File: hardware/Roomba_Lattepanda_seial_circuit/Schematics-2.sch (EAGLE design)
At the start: 14 parts

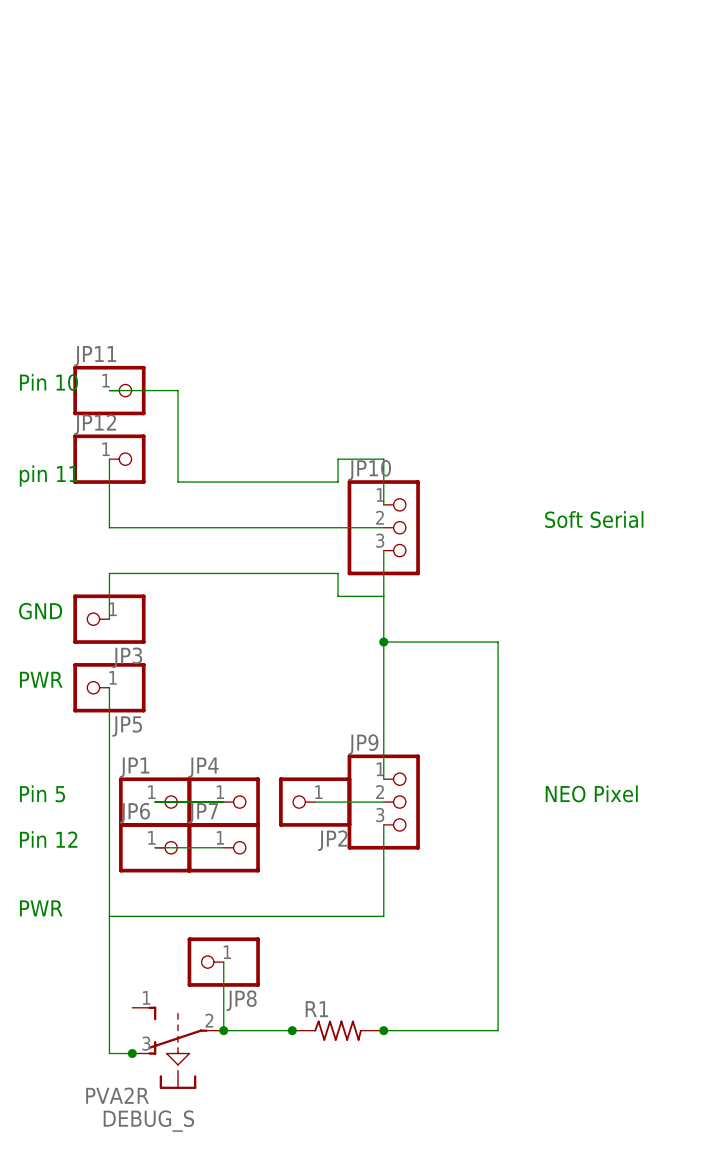
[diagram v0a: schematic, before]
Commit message: update hardware
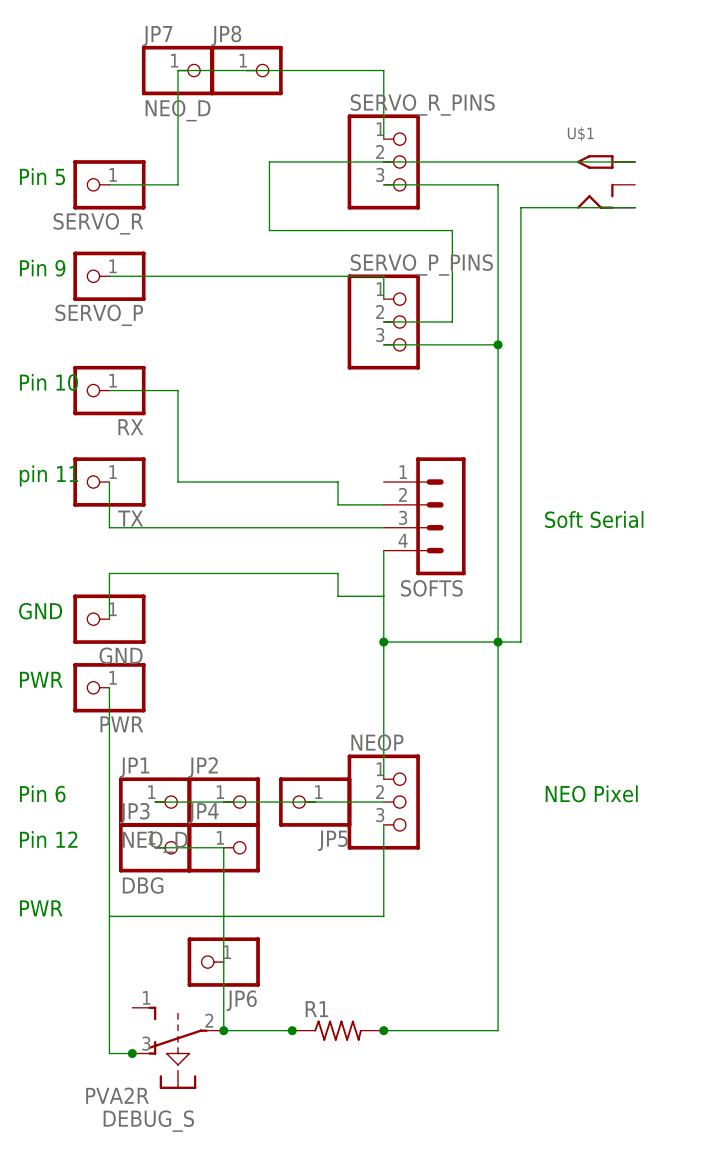
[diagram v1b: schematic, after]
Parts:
- removed JP10: (no value), adafruit:PINHD-1X3CB
- removed JP11, JP12: (no value), adafruit:PINHD-1X1
- added GND, PWR, RX, SERVO_P, SERVO_R, TX: (no value), adafruit:PINHD-1X1CB
- added SERVO_P_PINS, SERVO_R_PINS: (no value), adafruit:PINHD-1X3CB
- added SOFTS: (no value), con-lstb:MA04-1
- added U$1: 2.1MMJACKTHM, adafruit:2.1MMJACKTHM
- JP1, JP7: value (none) -> NEO_D
- JP3: value (none) -> DBG
- renumbered JP9 to NEOP
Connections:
- removed net N$6: DEBUG_S1.P, JP8.1, R1.1
- removed net N$7: JP2.1, NEOP.2
- new net N$10: JP7.1, JP8.1, SERVO_R.1, SERVO_R_PINS.1
- new net N$12: SERVO_P.1, SERVO_P_PINS.1
- new net N$9: SERVO_P_PINS.2, SERVO_R_PINS.2, U$1.TIP
- net N$1: now also RX.1, SOFTS.2; no longer JP10.1, JP11.1
- net N$2: now also JP2.1, JP5.1, NEOP.2; no longer JP4.1
- net N$3: now also SOFTS.3, TX.1; no longer JP10.2, JP12.1
- net N$4: now also GND.1, SERVO_P_PINS.3, SERVO_R_PINS.3, SOFTS.4, U$1.RING; no longer JP10.3, JP3.1
- net N$5: now also PWR.1; no longer JP5.1
- net N$8: now also DEBUG_S1.P, JP3.1, JP4.1, R1.1; no longer JP7.1
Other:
- note added: "Pin 6"
- note added: "Pin 9"
- moved on the sheet: JP2, JP3, JP4, JP5, JP6, JP7, JP8
